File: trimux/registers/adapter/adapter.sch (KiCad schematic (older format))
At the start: 20 parts, among them P1 CONN_02X05, P10 CONN_02X05, P11 CONN_02X05, P12 CONN_02X05, P13 CONN_02X05, P2 CONN_02X05, P21 CONN_02X08, P22 CONN_02X08, P23 CONN_02X08, P24 CONN_02X08, P25 CONN_02X08, P26 CONN_02X08, P27 CONN_02X08, P3 CONN_02X05, P4 CONN_02X05, P5 CONN_02X05, P6 CONN_02X05, P7 CONN_02X05, P8 CONN_02X05, P9 CONN_02X05

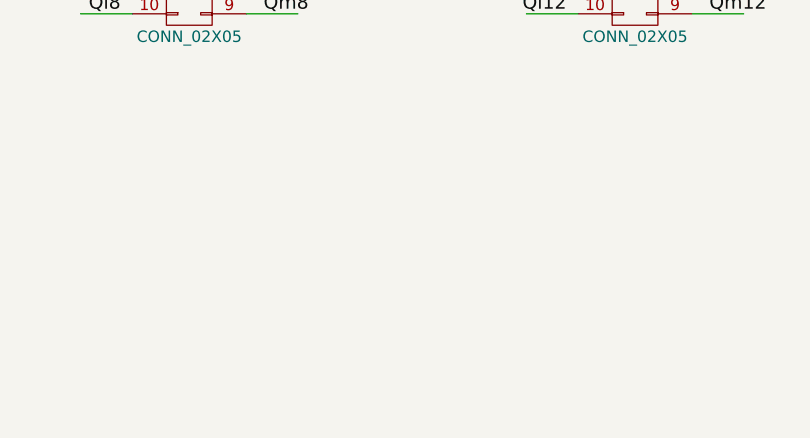
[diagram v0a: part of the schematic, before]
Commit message: memory
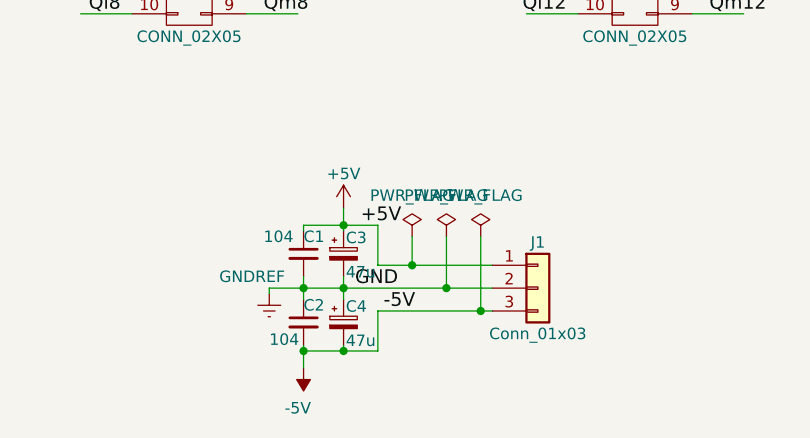
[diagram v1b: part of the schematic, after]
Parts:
- added C1, C2: 104, Capacitors_SMD:C_1206_HandSoldering, symbol C_Small
- added C3, C4: 47u, Capacitors_THT:CP_Radial_D5.0mm_P2.00mm, symbol CP_Small
- added J1: Conn_01x03, Pin_Headers:Pin_Header_Straight_1x03_Pitch2.54mm, symbol Conn_01x03
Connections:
- net labels added: GNDREF
- wire segments 254 -> 271
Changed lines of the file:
@@
 Wire Wire Line
 	10025 1025 9825 1025
+$Comp
+L GNDREF #PWR01
+U 1 1 59CBB376
+P 4025 5975
+F 0 "#PWR01" H 4025 5725 50  0001 C CNN
+F 1 "GNDREF" H 4100 6050 50  0000 C CNN
+F 2 "" H 4025 5975 50  0000 C CNN
+F 3 "" H 4025 5975 50  0000 C CNN
+	1    4025 5975
+	-1   0    0    -1
+$EndComp
+$Comp
+L -5V #PWR2
+U 1 1 59CBB37C
+P 4175 6300
+F 0 "#PWR2" H 4350 6275 50  0001 C CNN
+F 1 "-5V" H 4200 6475 50  0000 C CNN
+F 2 "" H 4175 6300 50  0000 C CNN
+F 3 "" H 4175 6300 50  0000 C CNN
+	1    4175 6300
+	-1   0    0    1
+$EndComp
+$Comp
+L PWR_FLAG #FLG02
+U 1 1 59CBB382
+P 4650 5725
+F 0 "#FLG02" H 4650 5820 50  0001 C CNN
+F 1 "PWR_FLAG" H 4650 5905 50  0000 C CNN
+F 2 "" H 4650 5725 50  0000 C CNN
+F 3 "" H 4650 5725 50  0000 C CNN
+	1    4650 5725
+	-1   0    0    -1
+$EndComp
+$Comp
+L PWR_FLAG #FLG03
+U 1 1 59CBB388
+P 4950 5725
+F 0 "#FLG03" H 4950 5820 50  0001 C CNN
+F 1 "PWR_FLAG" H 4950 5905 50  0000 C CNN
+F 2 "" H 4950 5725 50  0000 C CNN
+F 3 "" H 4950 5725 50  0000 C CNN
+	1    4950 5725
+	-1   0    0    -1
+$EndComp
+$Comp
+L PWR_FLAG #FLG04
+U 1 1 59CBB38E
+P 4800 5725
+F 0 "#FLG04" H 4800 5820 50  0001 C CNN
+F 1 "PWR_FLAG" H 4800 5905 50  0000 C CNN
+F 2 "" H 4800 5725 50  0000 C CNN
+F 3 "" H 4800 5725 50  0000 C CNN
+	1    4800 5725
+	-1   0    0    -1
+$EndComp
+$Comp
+L CP_Small C3
+U 1 1 59CBB394
+P 4350 5800
+F 0 "C3" H 4360 5870 50  0000 L CNN
+F 1 "47u" H 4360 5720 50  0000 L CNN
+F 2 "Capacitors_THT:CP_Radial_D5.0mm_P2.00mm" H 4350 5800 50  0001 C CNN
+F 3 "" H 4350 5800 50  0000 C CNN
+	1    4350 5800
+	1    0    0    -1
+$EndComp
+$Comp
+L CP_Small C4
+U 1 1 59CBB39B
+P 4350 6100
+F 0 "C4" H 4360 6170 50  0000 L CNN
+F 1 "47u" H 4360 6020 50  0000 L CNN
+F 2 "Capacitors_THT:CP_Radial_D5.0mm_P2.00mm" H 4350 6100 50  0001 C CNN
+F 3 "" H 4350 6100 50  0000 C CNN
+	1    4350 6100
+	1    0    0    -1
+$EndComp
+$Comp
+L +5V #PWR05
+U 1 1 59CBB3A2
+P 4350 5600
+F 0 "#PWR05" H 4350 5450 50  0001 C CNN
+F 1 "+5V" H 4350 5750 50  0000 C CNN
+F 2 "" H 4350 5600 50  0000 C CNN
+F 3 "" H 4350 5600 50  0000 C CNN
+	1    4350 5600
+	-1   0    0    -1
+$EndComp
+$Comp
+L C_Small C1
+U 1 1 59CBB3A8
+P 4175 5800
+F 0 "C1" H 4175 5875 50  0000 L CNN
+F 1 "104" H 4000 5875 50  0000 L CNN
+F 2 "Capacitors_SMD:C_1206_HandSoldering" H 4175 5800 50  0001 C CNN
+F 3 "" H 4175 5800 50  0000 C CNN
+	1    4175 5800
+	1    0    0    -1
+$EndComp
+$Comp
+L C_Small C2
+U 1 1 59CBB3AF
+P 4175 6100
+F 0 "C2" H 4175 6175 50  0000 L CNN
+F 1 "104" H 4025 6025 50  0000 L CNN
+F 2 "Capacitors_SMD:C_1206_HandSoldering" H 4175 6100 50  0001 C CNN
+F 3 "" H 4175 6100 50  0000 C CNN
+	1    4175 6100
+	1    0    0    -1
+$EndComp
+Wire Wire Line
+	4025 5950 5000 5950
+Wire Wire Line
+	4350 5900 4350 6000
+Connection ~ 4350 5950
+Wire Wire Line
+	4500 6050 5000 6050
+Wire Wire Line
+	4500 6225 4500 6050
+Wire Wire Line
+	4500 5675 4500 5850
+Wire Wire Line
+	4500 5850 5000 5850
+Wire Wire Line
+	4025 5975 4025 5950
+Wire Wire Line
+	4175 6225 4500 6225
+Wire Wire Line
+	4350 6225 4350 6200
+Connection ~ 4350 6225
+Wire Wire Line
+	4350 5700 4350 5600
+Wire Wire Line
+	4650 5725 4650 5850
+Connection ~ 4650 5850
+Wire Wire Line
+	4800 5725 4800 5950
+Connection ~ 4800 5950
+Wire Wire Line
+	4950 5725 4950 6050
+Connection ~ 4950 6050
+Wire Wire Line
+	4175 5675 4500 5675
+Connection ~ 4350 5675
+Wire Wire Line
+	4175 5675 4175 5700
+Wire Wire Line
+	4175 5900 4175 6000
+Connection ~ 4175 5950
+Wire Wire Line
+	4175 6200 4175 6300
+$Comp
+L Conn_01x03 J1
+U 1 1 59CBB559
+P 5200 5950
+F 0 "J1" H 5200 6150 50  0000 C CNN
+F 1 "Conn_01x03" H 5200 5750 50  0000 C CNN
+F 2 "Pin_Headers:Pin_Header_Straight_1x03_Pitch2.54mm" H 5200 5950 50  0001 C CNN
+F 3 "" H 5200 5950 50  0001 C CNN
+	1    5200 5950
+	1    0    0    -1
+$EndComp
+Connection ~ 4175 6225
+Text Label 4425 5675 0    60   ~ 0
++5V
+Text Label 4400 5950 0    60   ~ 0
+GND
+Text Label 4525 6050 0    60   ~ 0
+-5V
 $EndSCHEMATC
